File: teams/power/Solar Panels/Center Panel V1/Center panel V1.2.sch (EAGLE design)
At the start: 7 parts

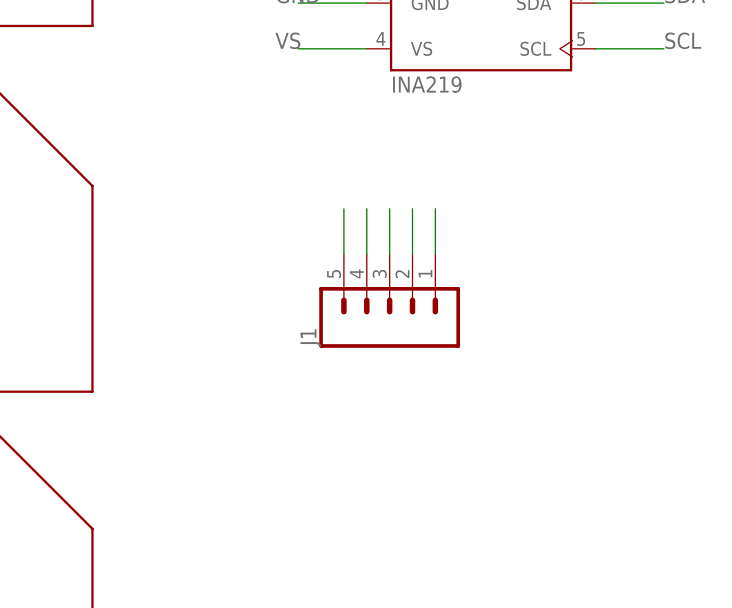
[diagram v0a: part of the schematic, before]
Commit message: Auto stash before merge of "develop" and "origin/develop"
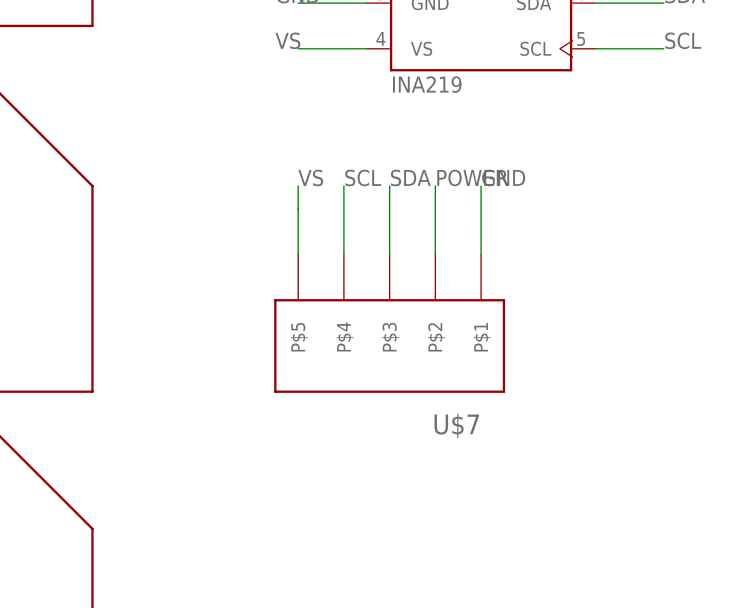
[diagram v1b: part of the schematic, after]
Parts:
- removed J1: (no value), SparkFun-Connectors:CONN_05SMD
- added U$7: PICOLOCK_5, DubSat1 Components:PICOLOCK_5
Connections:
- removed net N$11: J1.3
- removed net N$12: J1.4
- removed net N$13: J1.5
- net GND: now also U$7.P$1; no longer J1.1
- net POWER: now also U$7.P$2; no longer J1.2
- net SCL: now also U$7.P$4
- net SDA: now also U$7.P$3
- net VS: now also U$7.P$5
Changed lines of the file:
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@@
 <?xml version="1.0" encoding="utf-8"?>
 <!DOCTYPE eagle SYSTEM "eagle.dtd">
-<eagle version="7.6.0">
+<eagle version="8.3.1">
 <drawing>
 <settings>
 <setting alwaysvectorfont="no"/>
+<setting keepoldvectorfont="yes"/>
 <setting verticaltext="up"/>
 </settings>
@@
 <classes>
 <class number="0" name="default" width="0" drill="0">
+<clearance class="0" value="0.205"/>
 </class>
 </classes>
 <parts>
-<part name="U$1" library="DubSat1 Components" deviceset="SOLAR_CELL_BOTTOM" device=""/>
-<part name="U$2" library="DubSat1 Components" deviceset="SOALAR_CELL_OUTLINE" device=""/>
-<part name="U$3" library="DubSat1 Components" deviceset="SOALAR_CELL_OUTLINE" device=""/>
-<part name="U$5" library="DubSat1 Components" deviceset="SOLAR_CELL_TOP" device=""/>
-<part name="U$6" library="DubSat1 Components" deviceset="SOLAR_CELL_STAND-ALONE" device=""/>
+<part name="U$1" library="DubSat1 Components" library_urn="urn:adsk.eagle:library:348159" deviceset="SOLAR_CELL_BOTTOM" device="" package3d_urn="urn:adsk.eagle:package:348282/2"/>
+<part name="U$2" library="DubSat1 Components" library_urn="urn:adsk.eagle:library:348159" deviceset="SOALAR_CELL_OUTLINE" device="" package3d_urn="urn:adsk.eagle:package:348279/2"/>
+<part name="U$3" library="DubSat1 Components" library_urn="urn:adsk.eagle:library:348159" deviceset="SOALAR_CELL_OUTLINE" device="" package3d_urn="urn:adsk.eagle:package:348279/2"/>
+<part name="U$5" library="DubSat1 Components" library_urn="urn:adsk.eagle:library:348159" deviceset="SOLAR_CELL_TOP" device="" package3d_urn="urn:adsk.eagle:package:348280/2"/>
+<part name="U$6" library="DubSat1 Components" library_urn="urn:adsk.eagle:library:348159" deviceset="SOLAR_CELL_STAND-ALONE" device="" package3d_urn="urn:adsk.eagle:package:348283/2"/>
 <part name="GND1" library="SparkFun-PowerSymbols" deviceset="GND" device=""/>
-<part name="U$4" library="DubSat1 Components" deviceset="INA219" device=""/>
-<part name="J1" library="SparkFun-Connectors" deviceset="CONN_05" device="SMD"/>
+<part name="U$4" library="DubSat1 Components" library_urn="urn:adsk.eagle:library:348159" deviceset="INA219" device="" package3d_urn="urn:adsk.eagle:package:348285/2"/>
+<part name="U$7" library="DubSat1 Components" library_urn="urn:adsk.eagle:library:348159" deviceset="PICOLOCK_5" device="" package3d_urn="urn:adsk.eagle:package:348289/2"/>
 </parts>
 <sheets>
@@
 <instance part="GND1" gate="1" x="33.02" y="-12.7"/>
 <instance part="U$4" gate="G$1" x="109.22" y="83.82"/>
-<instance part="J1" gate="G$1" x="99.06" y="45.72" rot="R90"/>
+<instance part="U$7" gate="G$1" x="96.52" y="48.26" rot="R180"/>
 </instances>
 <busses>
@@
 </segment>
 <segment>
-<pinref part="J1" gate="G$1" pin="1"/>
-<wire x1="104.14" y1="53.34" x2="104.14" y2="58.42" width="0.1524" layer="91"/>
+<pinref part="U$7" gate="G$1" pin="P$1"/>
+<wire x1="109.22" y1="53.34" x2="109.22" y2="60.96" width="0.1524" layer="91"/>
+<label x="109.22" y="60.96" size="1.778" layer="95"/>
 </segment>
 </net>
@@
 <label x="86.36" y="76.2" size="1.778" layer="95"/>
 </segment>
+<segment>
+<pinref part="U$7" gate="G$1" pin="P$5"/>
+<wire x1="88.9" y1="53.34" x2="88.9" y2="58.42" width="0.1524" layer="91"/>
+<wire x1="88.9" y1="60.96" x2="88.9" y2="58.42" width="0.1524" layer="91"/>
+<label x="88.9" y="60.96" size="1.778" layer="95"/>
+</segment>
 </net>
 <net name="SDA" class="0">
@@
 <label x="129.54" y="81.28" size="1.778" layer="95"/>
 </segment>
+<segment>
+<pinref part="U$7" gate="G$1" pin="P$3"/>
+<wire x1="99.06" y1="53.34" x2="99.06" y2="60.96" width="0.1524" layer="91"/>
+<label x="99.06" y="60.96" size="1.778" layer="95"/>
+</segment>
 </net>
 <net name="SCL" class="0">
@@
 <label x="129.54" y="76.2" size="1.778" layer="95"/>
 </segment>
+<segment>
+<pinref part="U$7" gate="G$1" pin="P$4"/>
+<wire x1="93.98" y1="53.34" x2="93.98" y2="60.96" width="0.1524" layer="91"/>
+<label x="93.98" y="60.96" size="1.778" layer="95"/>
+</segment>
 </net>
 <net name="POWER" class="0">
 <segment>
-<pinref part="J1" gate="G$1" pin="2"/>
-<wire x1="101.6" y1="53.34" x2="101.6" y2="58.42" width="0.1524" layer="91"/>
-</segment>
-</net>
-<net name="N$11" class="0">
-<segment>
-<pinref part="J1" gate="G$1" pin="3"/>
-<wire x1="99.06" y1="53.34" x2="99.06" y2="58.42" width="0.1524" layer="91"/>
-</segment>
-</net>
-<net name="N$12" class="0">
-<segment>
-<pinref part="J1" gate="G$1" pin="4"/>
-<wire x1="96.52" y1="53.34" x2="96.52" y2="58.42" width="0.1524" layer="91"/>
-</segment>
-</net>
-<net name="N$13" class="0">
-<segment>
-<pinref part="J1" gate="G$1" pin="5"/>
-<wire x1="93.98" y1="53.34" x2="93.98" y2="58.42" width="0.1524" layer="91"/>
+<pinref part="U$7" gate="G$1" pin="P$2"/>
+<wire x1="104.14" y1="53.34" x2="104.14" y2="60.96" width="0.1524" layer="91"/>
+<label x="104.14" y="60.96" size="1.778" layer="95"/>
 </segment>
 </net>
@@
 </schematic>
 </drawing>
+<compatibility>
+<note version="8.2" severity="warning">
+Since Version 8.2, EAGLE supports online libraries. The ids
+of those online libraries will not be understood (or retained)
+with this version.
+</note>
+<note version="8.3" severity="warning">
+Since Version 8.3, EAGLE supports URNs for individual library
+assets (packages, symbols, and devices). The URNs of those assets
+will not be understood (or retained) with this version.
+</note>
+<note version="8.3" severity="warning">
+Since Version 8.3, EAGLE supports the association of 3D packages
+with devices in libraries, schematics, and board files. Those 3D
+packages will not be understood (or retained) with this version.
+</note>
+</compatibility>
 </eagle>
